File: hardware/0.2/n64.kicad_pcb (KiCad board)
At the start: 2 copper layers, 101.5 x 52.3 mm, 46 parts, among them J1 , J2 Conn_01x05_Male, J3 Conn_01x03_Male, J4 Conn_02x08_Counter_Clockwise, J5 Conn_01x09_Male, U1 ICE40HX4K-TQ144, U2 ATtiny45-20PU, U3 S25FL064, U4 TLV73312PDBV, U5 IS42S16320D, U6 Multicomp_Oscillator, U7 Nintendo_64_Logo, U8 ATtiny45V-10PU

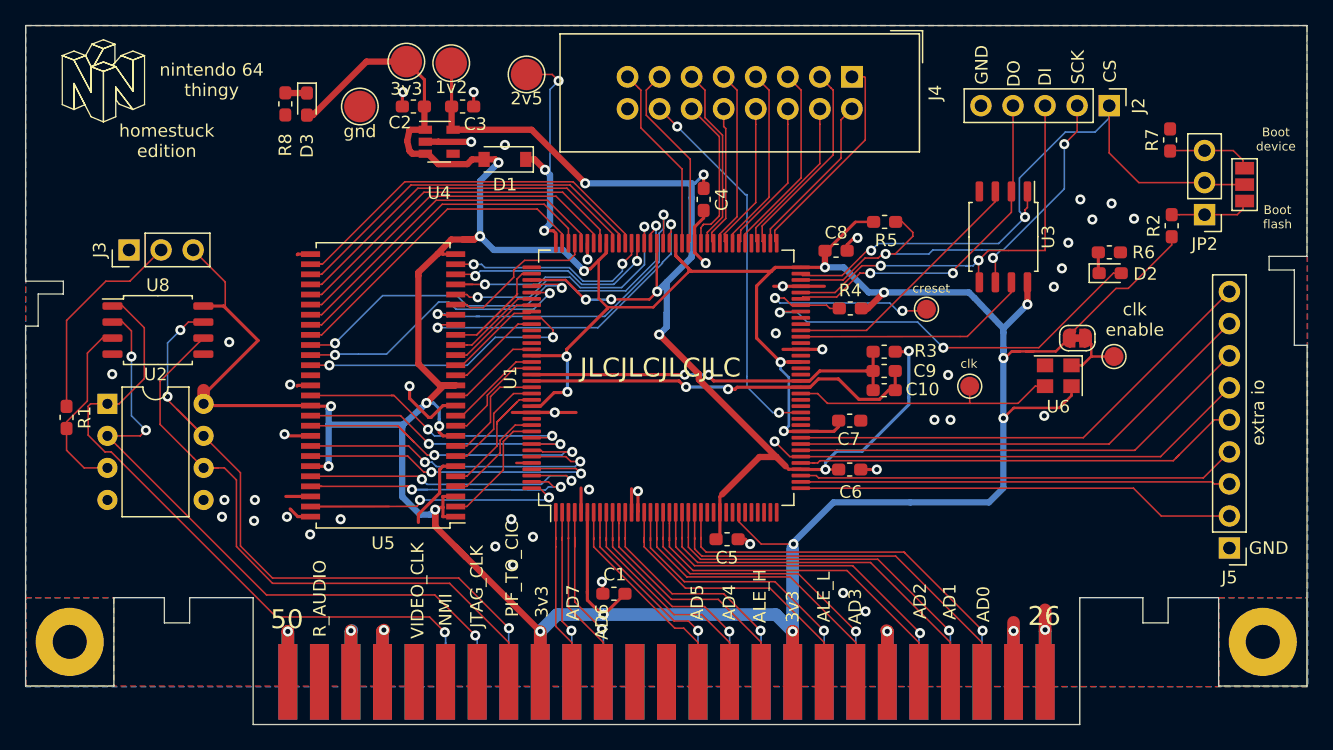
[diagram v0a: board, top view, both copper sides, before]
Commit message: some changes
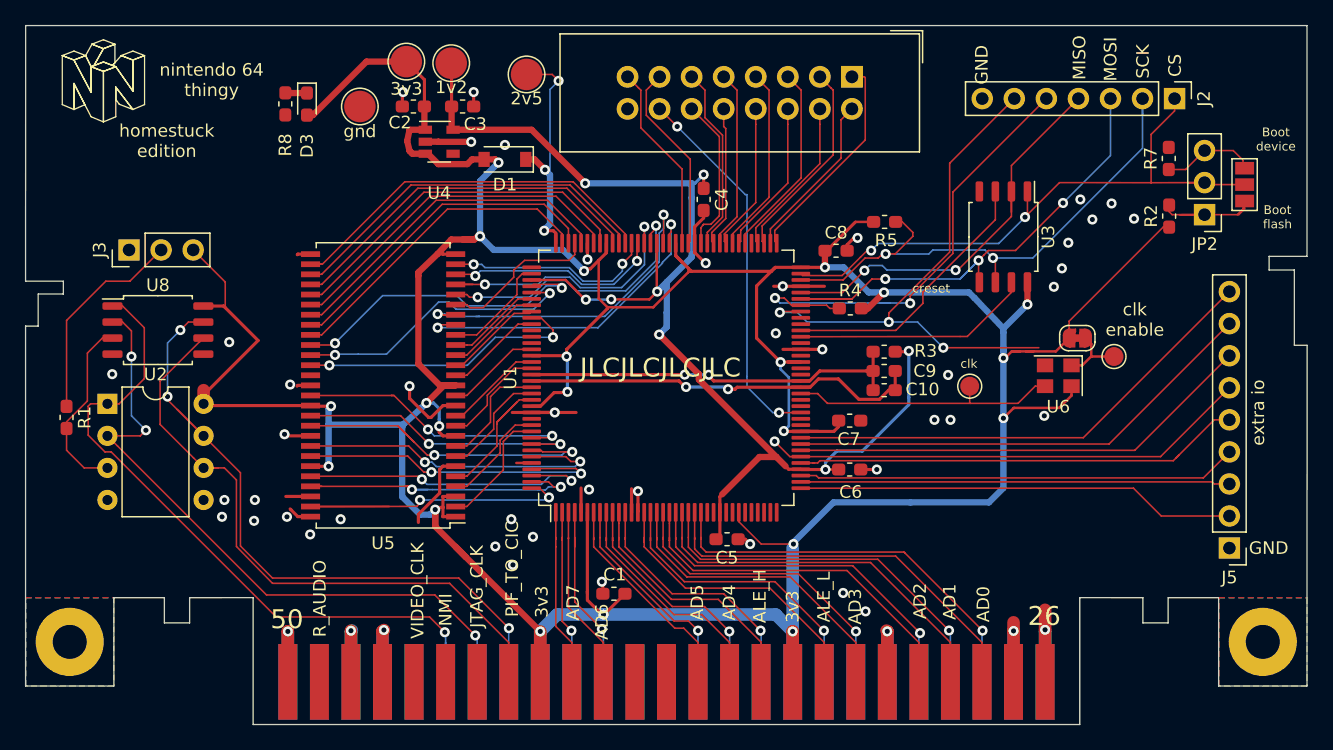
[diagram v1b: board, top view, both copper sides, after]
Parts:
- removed D2: LED, LED_SMD:LED_0603_1608Metric_Pad1.05x0.95mm_HandSolder
- removed R6: 1k, Resistor_SMD:R_0603_1608Metric_Pad1.05x0.95mm_HandSolder
- removed TP2: TestPoint, TestPoint:TestPoint_Pad_D1.5mm
- J2: value Conn_01x05_Male -> Conn_01x07_Male; footprint Connector_PinHeader_2.54mm:PinHeader_1x05_P2.54mm_Vertical -> Connector_PinHeader_2.54mm:PinHeader_1x07_P2.54mm_Vertical
- moved J2 5.21 mm to (171.9, 108.2)
- moved R7 1.47 mm to (171.4, 113.0)
- moved R2 0.79 mm to (171.4, 117.5)
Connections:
- net A12 renamed Net-(U1-Pad107)
- J2 pad 5: GND -> !CRESET
- R4 pad 1: Net-(R4-Pad1) -> !CRESET
- U1 pad 65: Net-(D2-Pad2) -> CDONE
- U1 pad 66: Net-(R4-Pad1) -> !CRESET
- U1 pad 67: FLASH_DO -> FLASH_DI
- U1 pad 68: FLASH_DI -> FLASH_DO
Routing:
- net CDONE: track 0.00 -> 45.2 mm, vias 0 -> 3
- net !CRESET: track 0.00 -> 37.8 mm, vias 0 -> 2
- net Net-(D2-Pad2): track 32.4 -> 0.00 mm, vias 2 -> 0
- net Net-(R4-Pad1): track 17.9 -> 0.00 mm, vias 2 -> 0
- net FLASH_DI: track 34.6 -> 42.4 mm, vias 2 -> 3
- net Net-(JP2-Pad1): track 6.34 -> 12.5 mm
- net FLASH_SCK: track 38.7 -> 44.0 mm, vias 3 -> 2
- net FLASH_DO: track 28.2 -> 33.0 mm
- net !CS: track 13.4 -> 8.75 mm
- net Net-(D2-Pad1): track 1.68 -> 0.00 mm
- net FLASH_CS: track 50.6 -> 49.2 mm
- net FLASH_IO2: track 20.4 -> 21.8 mm
- net +3V3: track 360.7 -> 362.0 mm
- net Net-(JP2-Pad3): track 6.79 -> 7.50 mm
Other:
- board text added: "MISO"
- board text added: "MOSI"
- board text removed: "DI"
- board text removed: "DO"
